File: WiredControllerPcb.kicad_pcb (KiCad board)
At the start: 2 copper layers, 91.4 x 45.7 mm, 35 parts, among them J1 Joystick, J2 Conn_01x06, J3 Conn_01x04, J4 Conn_01x06, J5 FlatCable, J6 Conn_01x05, J7 FlatCable, SW1 SW_Push, SW2 SW_Push, SW3 SW_Push, SW4 SW_Push, U1 LP2985-3.3, U2 ATmega328P-MU, Y1 8MHz

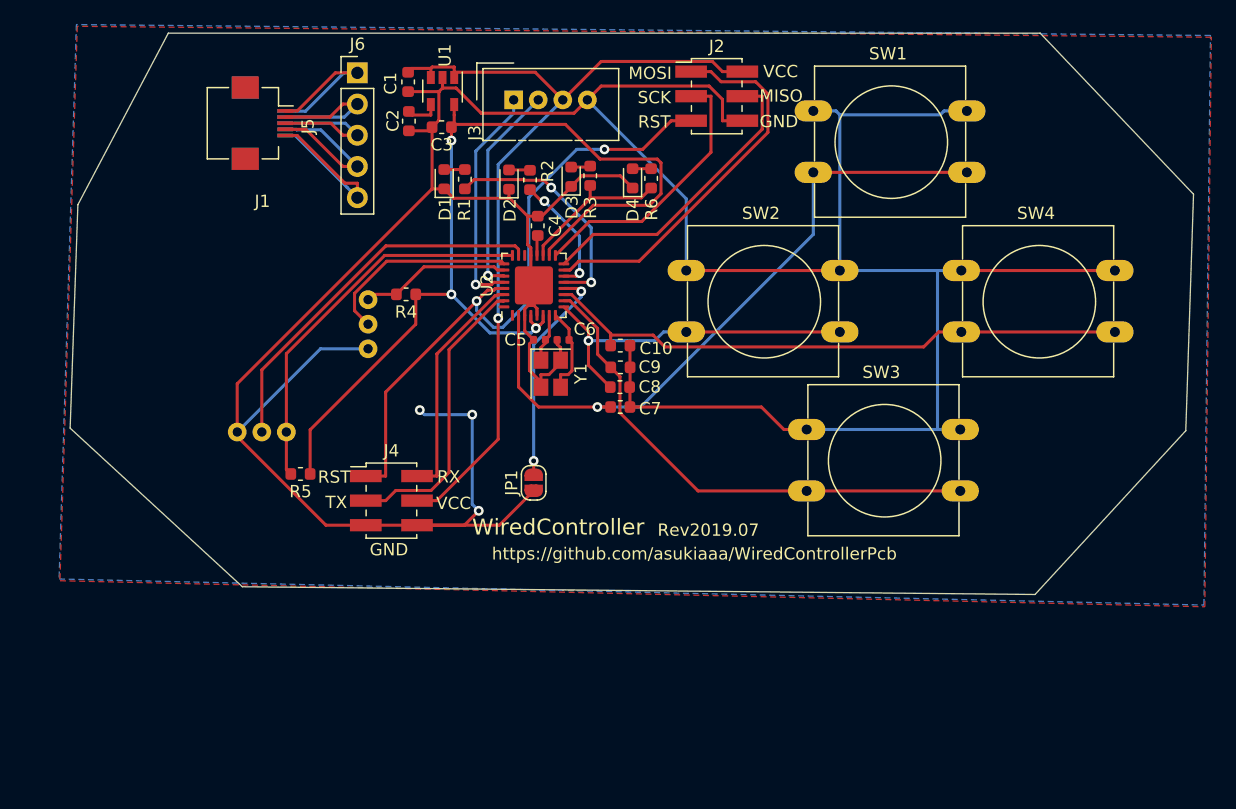
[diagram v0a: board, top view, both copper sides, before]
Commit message: Update pcb to order rev2019.08
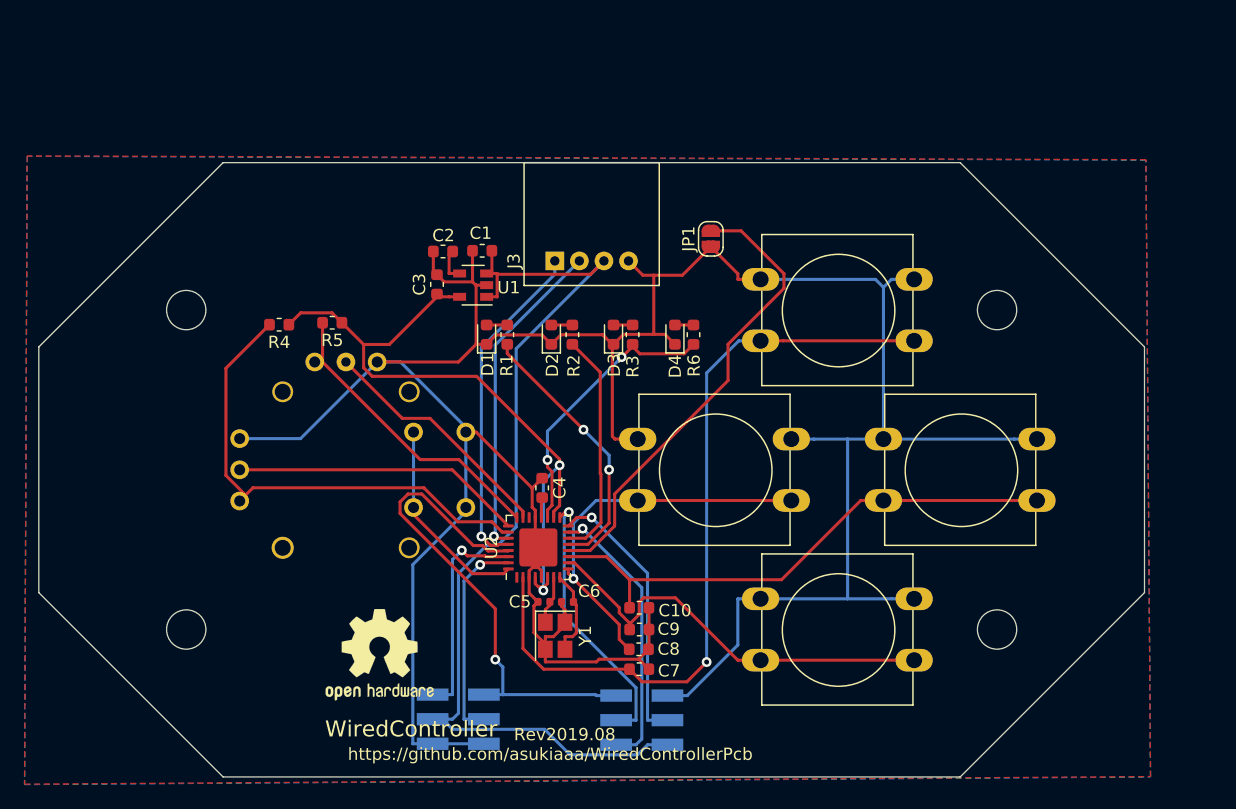
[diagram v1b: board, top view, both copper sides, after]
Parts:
- removed J5, J7: FlatCable, footprints:1x05-1MP_P0.50mm_Horizontal
- removed J6: Conn_01x05, Connector_PinHeader_2.54mm:PinHeader_1x05_P2.54mm_Vertical
- added REF**: OSHW-Logo2_9.8x8mm_SilkScreen, Symbol:OSHW-Logo2_9.8x8mm_SilkScreen, F.Cu at (127.7, 90.0)
- added REF1: MountingHole_3.2mm_M3, MountingHole:MountingHole_3.2mm_M3, F.Cu at (112.0, 62.0)
- added REF2: MountingHole_3.2mm_M3, MountingHole:MountingHole_3.2mm_M3, F.Cu at (112.0, 88.0)
- added REF3: MountingHole_3.2mm_M3, MountingHole:MountingHole_3.2mm_M3, F.Cu at (178.0, 62.0)
- added REF4: MountingHole_3.2mm_M3, MountingHole:MountingHole_3.2mm_M3, F.Cu at (178.0, 88.0)
- J1: footprint footprints:AdafruitJoystick -> footprints:PS4tJoystick
- J2, J4: moved to B.Cu
- J3: footprint Connector:NS-Tech_Grove_1x04_P2mm_Vertical -> footprints:NS-Tech_Grove_1x04_P2mm_Horizontal
- SW1, SW2, SW3, SW4: footprint Button_Switch_THT:SW_PUSH-12mm -> footprints:SW_Center_PUSH-12mm
- moved J2 51.2 mm to (149.1, 95.4)
- moved JP1 24.5 mm to (154.7, 56.2)
- moved C10 21.4 mm to (148.9, 86.2)
- moved C8 21.4 mm to (148.8, 89.6)
- moved C7 21.4 mm to (148.9, 91.2)
- moved C9 21.4 mm to (148.9, 88.0)
- moved C4 21.3 mm to (141.0, 76.5)
- moved C5 21.3 mm to (141.1, 85.8)
- moved C6 21.3 mm to (143.0, 85.8)
- moved Y1 21.3 mm to (142.0, 88.5)
- moved U2 21.3 mm to (140.7, 81.3)
- moved J4 18.6 mm to (134.1, 95.3), turned to 180 degrees
- moved SW3 16.5 mm to (165.0, 88.0)
- moved SW2 16.4 mm to (155.0, 75.0)
- moved SW1 16.3 mm to (165.0, 62.0)
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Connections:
- U2 pad 32: Net-(U2-Pad32) -> /JOY_PUSH
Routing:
- net GND: track 292.5 -> 252.1 mm, vias 3 -> 0
- net /VertFailSafe: track 12.3 -> 39.8 mm
- net +3V3: track 79.6 -> 56.3 mm, vias 3 -> 2
- net /ADDR: track 18.0 -> 38.2 mm, vias 2 -> 0
- net Net-(J5-Pad5): track 16.6 -> 0.00 mm
- net /JOY_PUSH: track 0.00 -> 16.6 mm
- net Net-(J5-Pad1): track 14.3 -> 0.00 mm
- net Net-(J5-Pad4): track 14.3 -> 0.00 mm
- net Net-(J5-Pad2): track 12.6 -> 0.00 mm
- net Net-(J5-Pad3): track 12.6 -> 0.00 mm
- net /RST: track 52.3 -> 41.0 mm, vias 2 -> 1
- net /HoriValue: track 30.8 -> 19.9 mm
- net /LED3: track 12.6 -> 22.8 mm, vias 0 -> 2
- net /SDA: track 17.3 -> 26.5 mm
- net /BTNT: track 54.9 -> 64.0 mm
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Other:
- board size 91.4 x 45.7 mm -> 90 x 50 mm
- board text added: "Rev2019.08"
- board text removed: "Rev2019.07"
